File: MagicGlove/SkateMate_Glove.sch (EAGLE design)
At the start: 45 parts, among them IC1 BU33TD3WG, IC2 LMV321M5, U2 ATMEGA328PB-AU

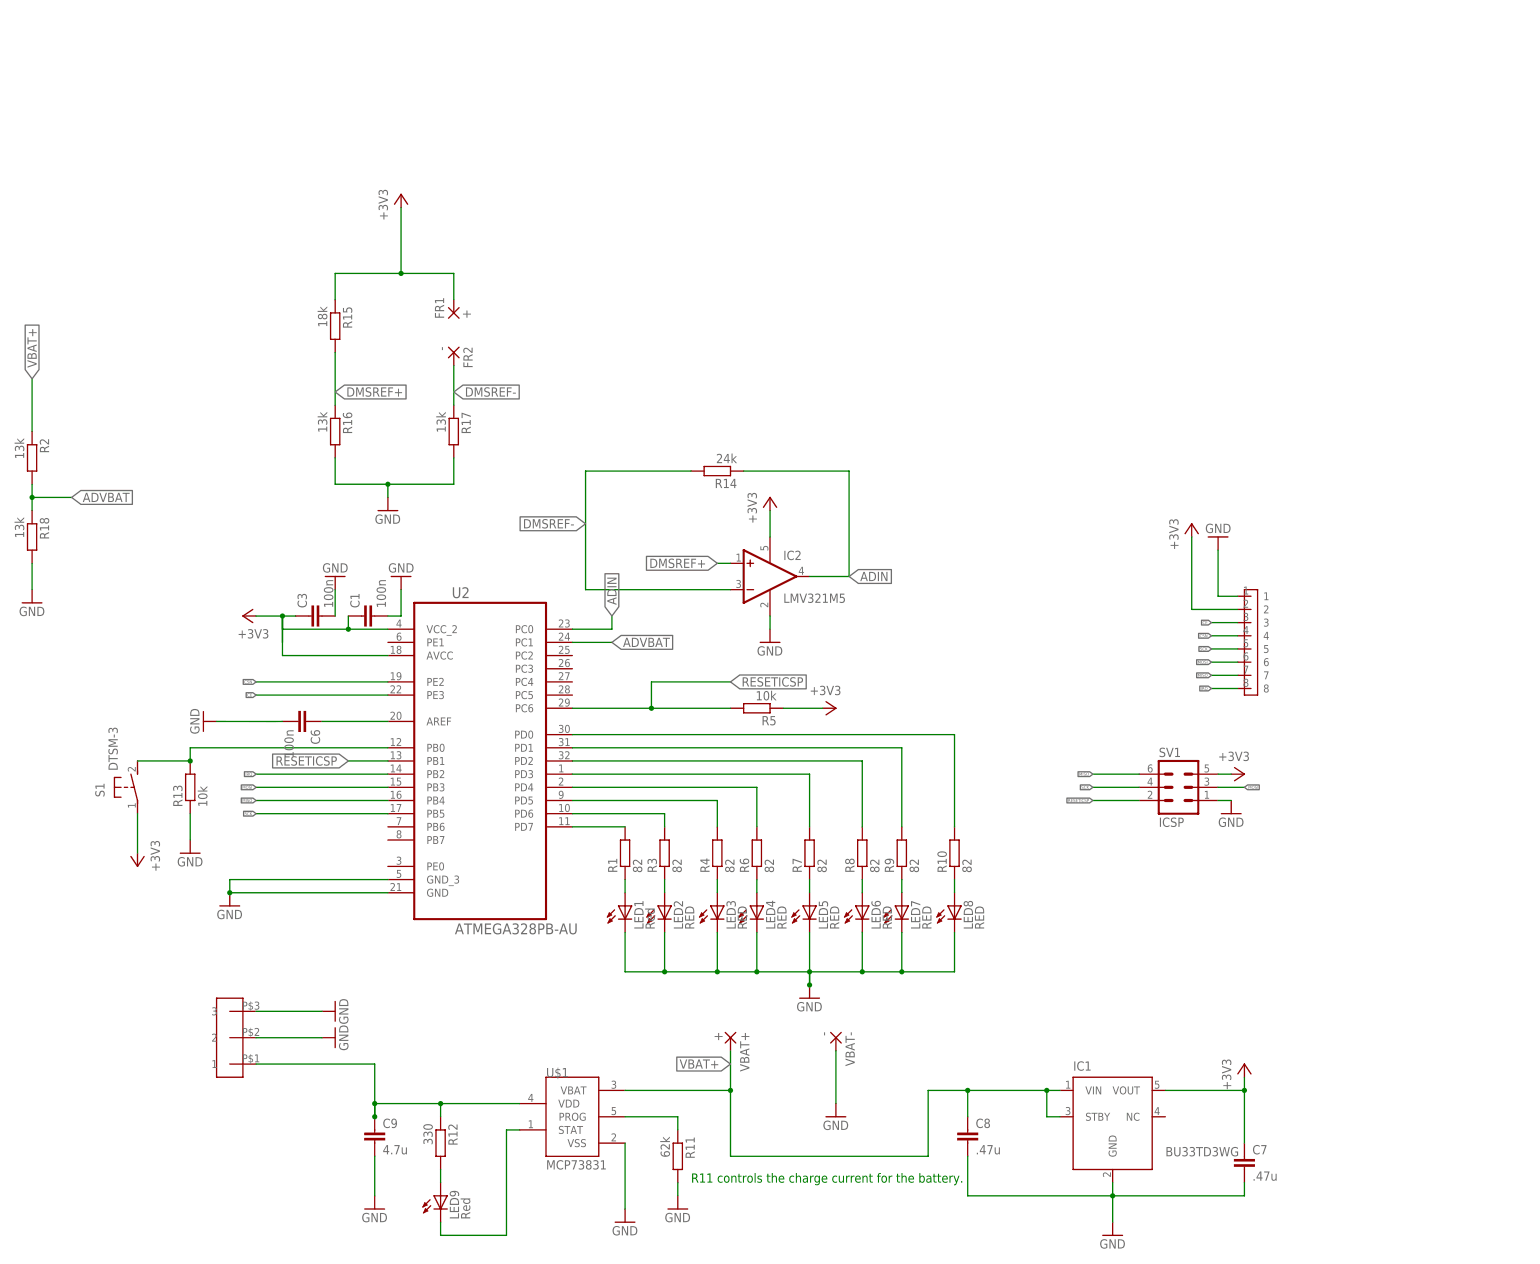
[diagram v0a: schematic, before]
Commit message: style
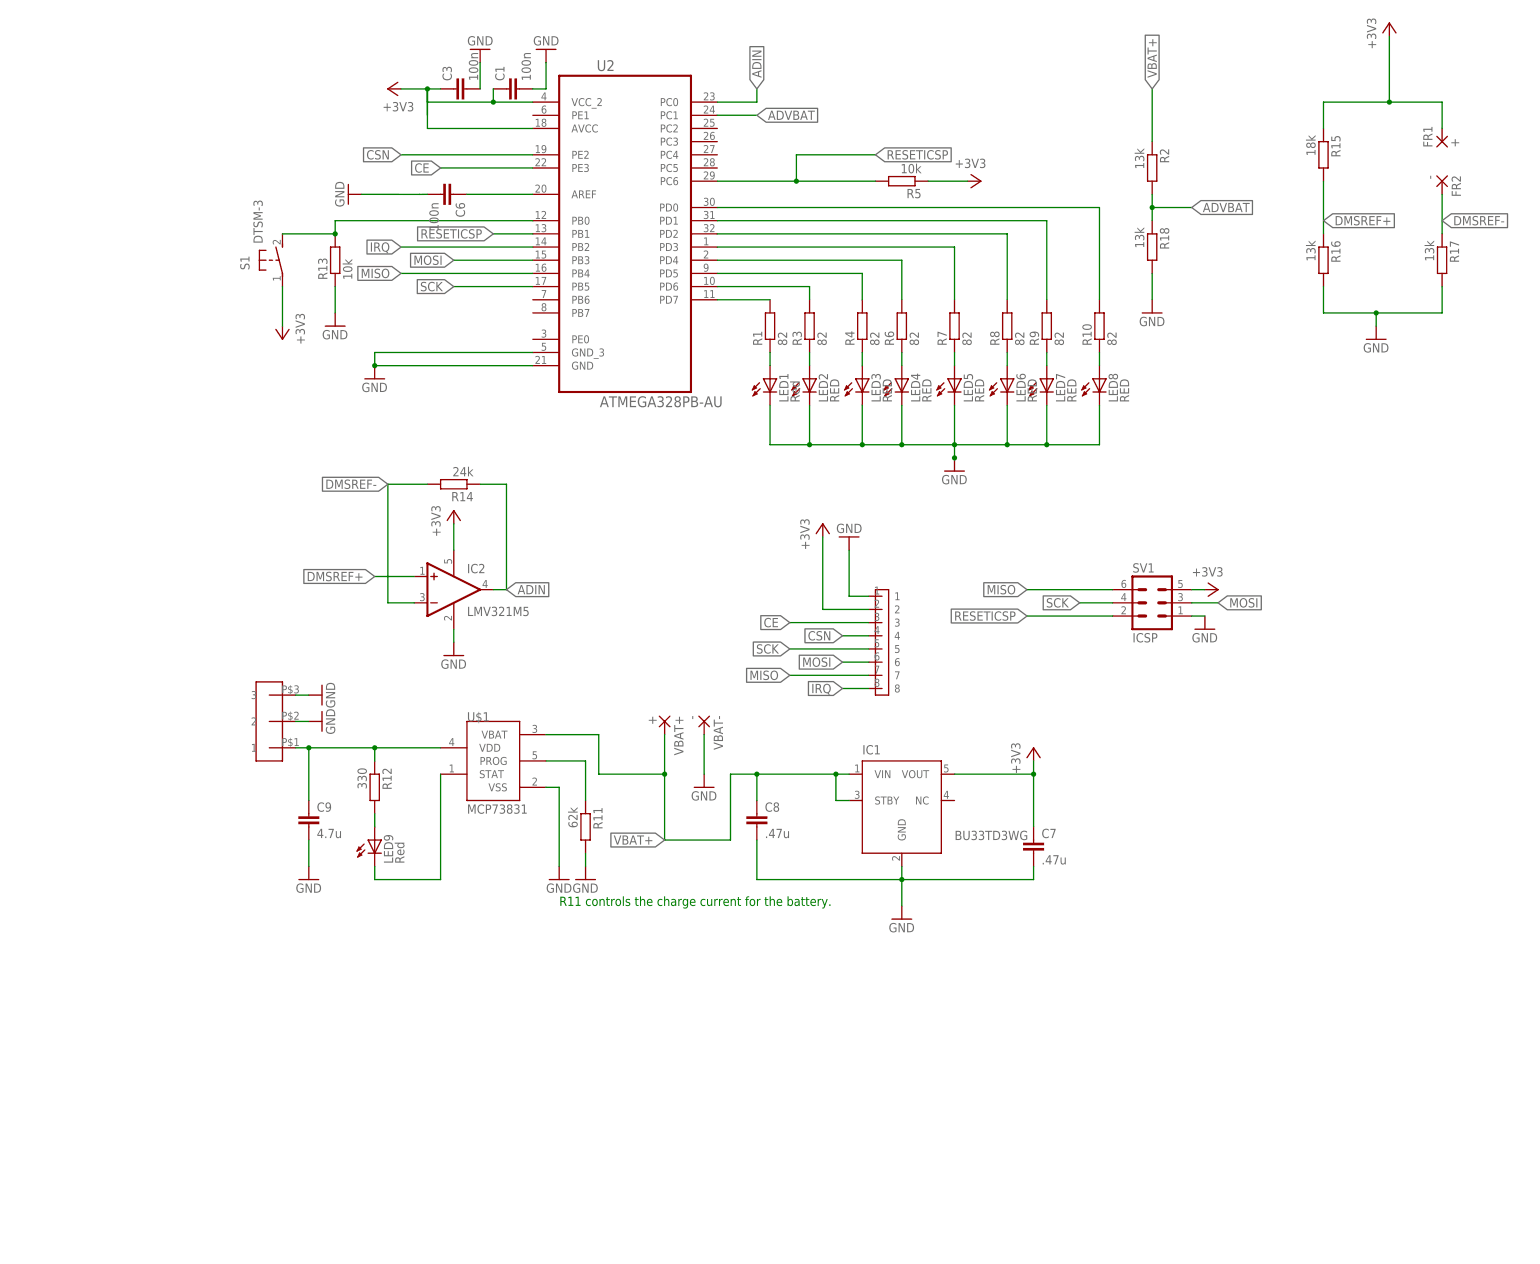
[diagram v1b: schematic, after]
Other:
- moved on the sheet: C1, C3, C6, C7, C8, C9, FR1, FR2, IC1, IC2, LED1, LED2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
